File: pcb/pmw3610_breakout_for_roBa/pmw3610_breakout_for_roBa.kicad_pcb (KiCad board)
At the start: 2 copper layers, 22 x 23.5 mm, 13 parts, among them J2 vik-module-connector, U1 MCP1700T-1802E/TT, U2 PMW3610

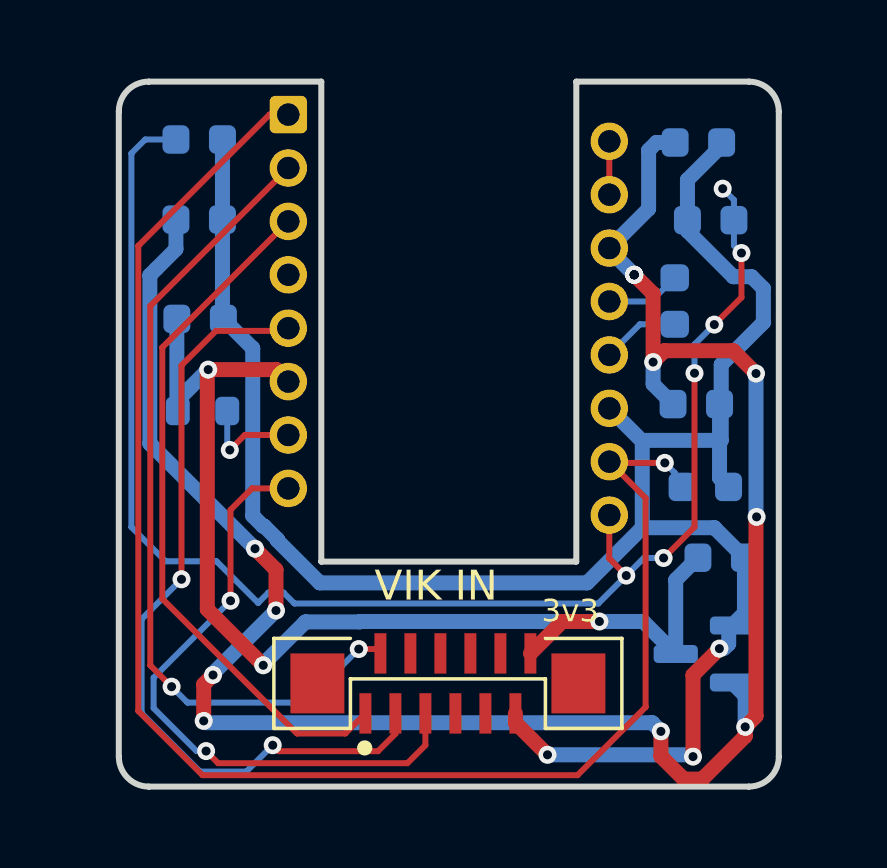
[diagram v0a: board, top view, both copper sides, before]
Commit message: Update pmw3610 breakout
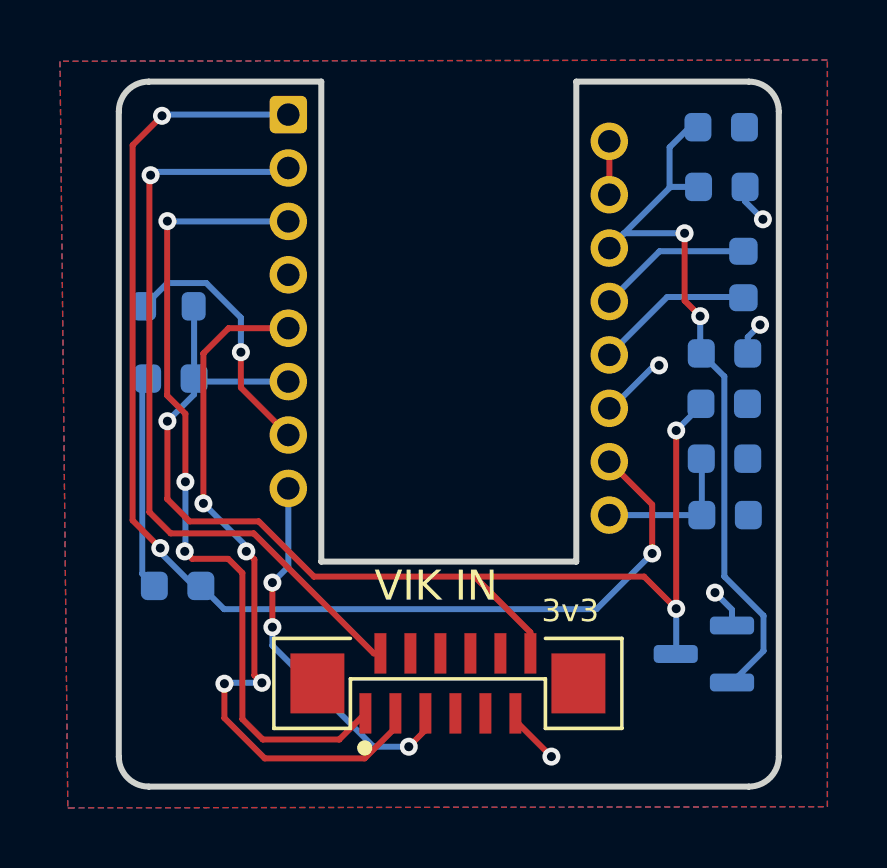
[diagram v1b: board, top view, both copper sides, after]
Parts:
- moved C7 20.5 mm to (145.2, 92.6)
- moved C2 18.1 mm to (145.2, 89.1)
- moved C4 17.9 mm to (127.0, 96.8), turned to 180 degrees
- moved C6 9.84 mm to (145.2, 94.5), turned to 0 degrees
- moved C9 7.29 mm to (145.1, 83.5)
- moved C1 5.13 mm to (145.2, 90.7)
- moved R1 3.67 mm to (126.7, 87.5), turned to 0 degrees
- moved C5 2.46 mm to (145.8, 86.4)
- moved C3 2.22 mm to (126.7, 89.9), turned to 180 degrees
- moved C8 0.92 mm to (145.1, 81.5)
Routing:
- net GND: track 68.6 -> 15.1 mm, vias 3 -> 5
- net Net-(U2-VCP): track 49.8 -> 5.01 mm, vias 6 -> 0
- net +1V9: track 68.4 -> 25.7 mm, vias 12 -> 2
- net Net-(U2-+VCSEL): track 52.3 -> 41.2 mm, vias 1 -> 3
- net MOTION: track 21.1 -> 12.7 mm, vias 2 -> 3
- net Net-(U2-NRESET): track 3.49 -> 8.60 mm
- net SCLK: track 23.2 -> 27.1 mm, vias 0 -> 3
- net Net-(U2-CP): track 2.60 -> 5.28 mm
- net Net-(U2-CN): track 2.64 -> 5.16 mm
- net NCS: track 26.9 -> 24.5 mm, vias 2 -> 4
- net SDIO: track 27.5 -> 25.7 mm, vias 2 -> 1
- net VCC: track 39.4 -> 40.6 mm
- added copper zone on B.Cu, net GND
- added copper zone on F.Cu, net GND
